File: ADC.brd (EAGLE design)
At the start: 132.1 x 82.5 mm, 368 parts, among them IC1 AD8221ARZ, IC10 AD8605ARTZ, IC11 AD8221ARZ, IC12 TLC2254ID, IC13 AD8605ARTZ, IC14 AD8221ARZ, IC15 TLC2254ID, IC16 AD8605ARTZ, IC17 AD8221ARZ, IC18 TLC2254ID, IC19 AD8605ARTZ, IC2 TLC2254ID, IC20 AD8221ARZ, IC21 TLC2254ID, IC22 AD8605ARTZ, IC23 AD8221ARZ, IC24 TLC2254ID, IC25 AD8605ARTZ, IC26 AD8221ARZ, IC27 TLC2254ID, IC28 AD8605ARTZ, IC3 ADS1256IDBT, IC4 AD8605ARTZ, IC5 MCP170333MB, IC6 ADUM1402ARWZ, IC7 REF3125AIDBZT, IC8 AD8221ARZ, IC9 TLC2254ID, Q1 8MHz

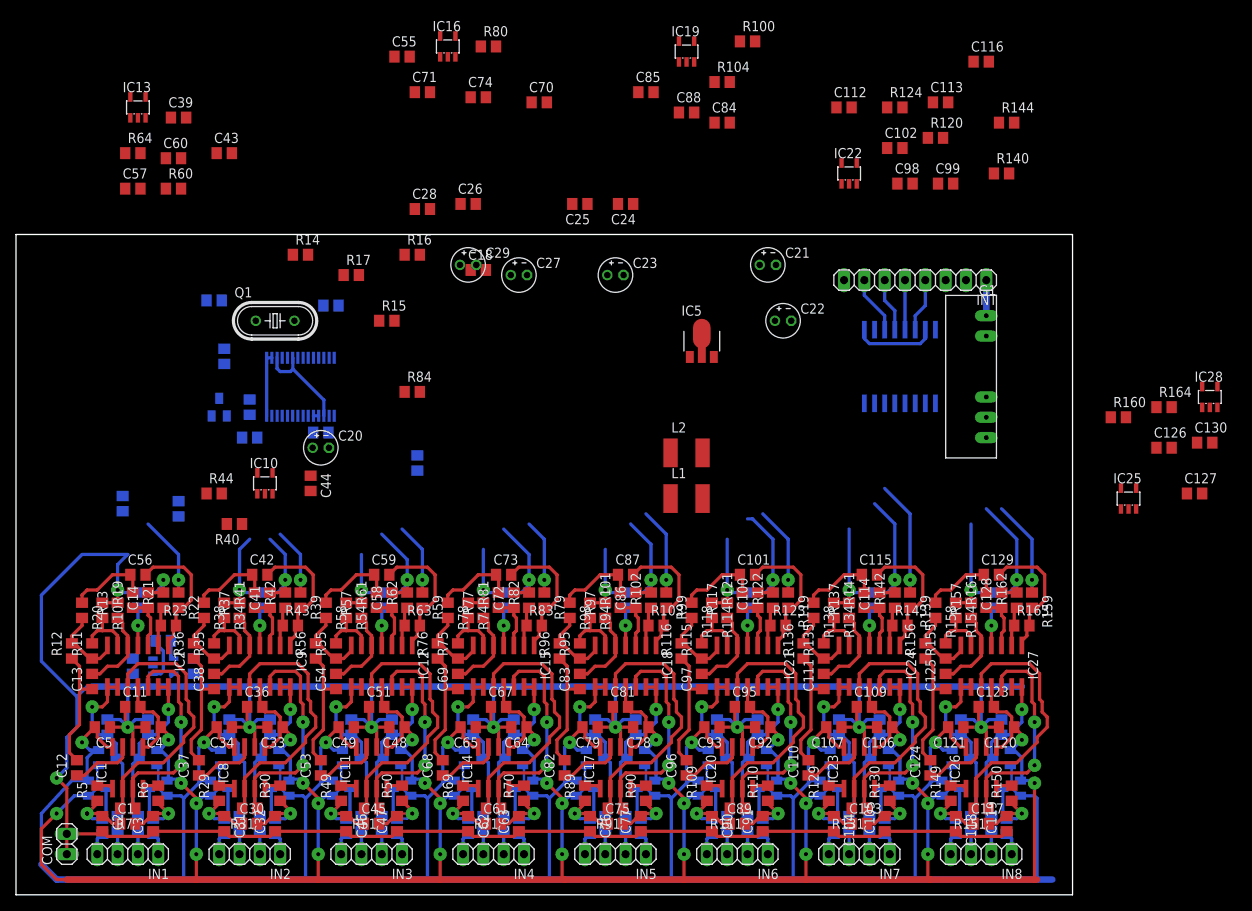
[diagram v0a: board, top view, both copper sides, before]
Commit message: Latest modification for all-in-one board
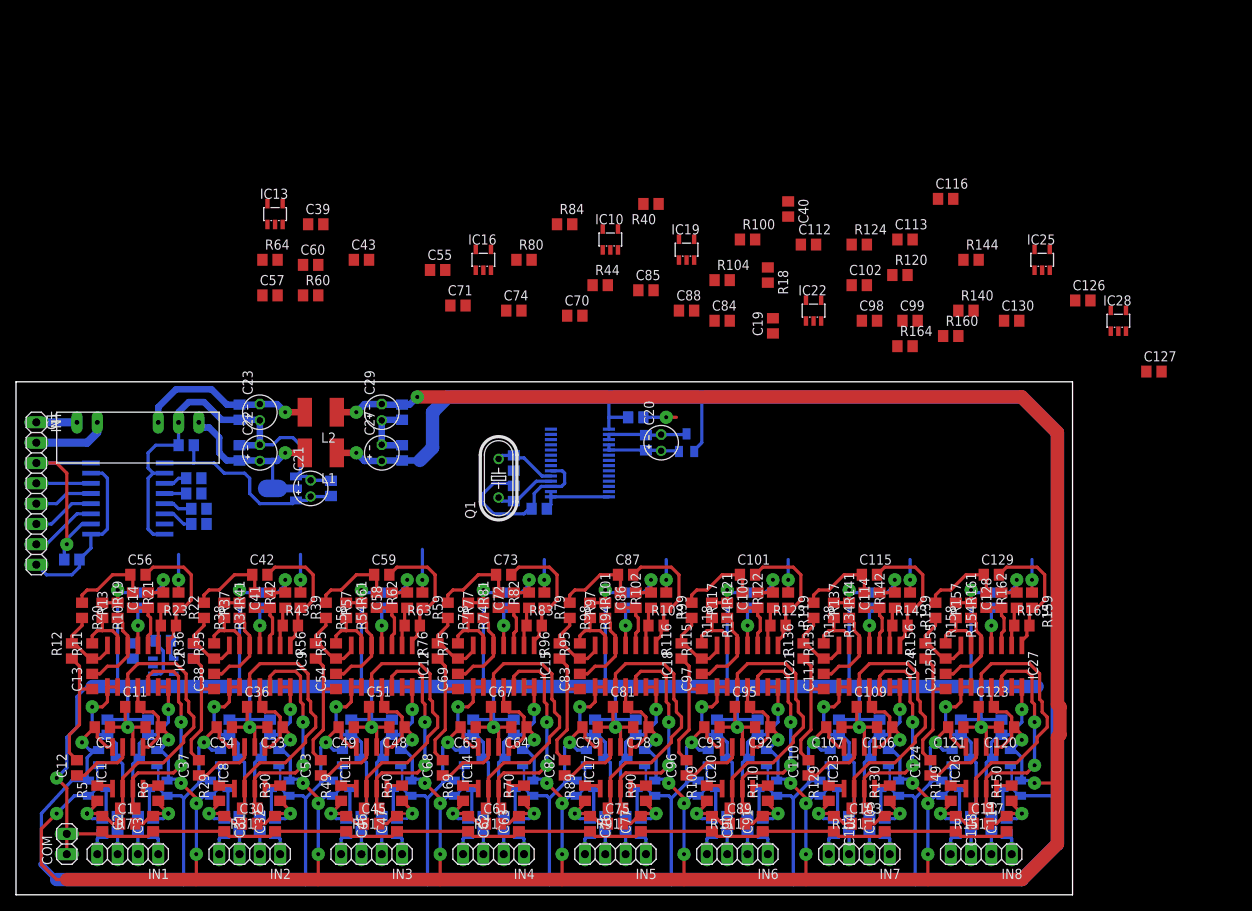
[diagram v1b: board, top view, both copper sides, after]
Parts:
- moved INT 113.0 mm to (2.54, 50.2), turned to 270 degrees
- moved G1 106.2 mm to (15.2, 59.1), turned to 90 degrees
- moved IC6 97.9 mm to (14.0, 49.5), turned to 270 degrees
- moved C19 84.3 mm to (94.6, 71.1), flipped to the top
- moved R18 79.2 mm to (94.0, 77.5), flipped to the top
- moved C22 67.5 mm to (30.5, 55.2), turned to 90 degrees
- moved R40 65.7 mm to (79.4, 86.4)
- moved C21 63.6 mm to (36.8, 50.8), turned to 90 degrees
- moved C18 62.4 mm to (6.99, 41.9), flipped to the bottom, turned to 180 degrees
- moved IC7 58.6 mm to (83.8, 56.5)
- moved C24 57.4 mm to (27.9, 55.2), flipped to the bottom, turned to 90 degrees
- moved C40 56.2 mm to (96.5, 85.7), flipped to the top, turned to 270 degrees
- moved IC5 55.8 mm to (33.0, 50.8), flipped to the bottom, turned to 270 degrees
- moved R44 54.8 mm to (73.0, 76.2)
- moved IC10 52.9 mm to (74.3, 81.9)
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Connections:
- new net N$207: G1.2, INT.2
- net N$37: no longer G1.2, INT.3
- net N$38: now also INT.3; no longer INT.2
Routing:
- net +5VA: track 458.4 -> 616.0 mm, vias 16 -> 17
- net -5VA: track 460.6 -> 599.9 mm, vias 31 -> 33
- net GND: track 685.2 -> 730.5 mm, vias 25 -> 26
- net +3.3V: track 7.90 -> 36.2 mm
- net N$38: track 0.00 -> 26.5 mm, vias 0 -> 1
- net N$44: track 0.00 -> 22.4 mm, vias 0 -> 1
- net N$39: track 0.00 -> 20.2 mm, vias 0 -> 1
- net N$37: track 10.4 -> 22.0 mm
- net N$178: track 14.3 -> 4.13 mm
- net N$207: track 0.00 -> 9.42 mm
- net VREF: track 0.65 -> 9.49 mm
- net N$202: track 12.1 -> 4.13 mm
- net N$13: track 0.00 -> 7.78 mm
- net N$12: track 0.00 -> 7.75 mm
- net N$155: track 11.2 -> 4.13 mm
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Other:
- board size 132.1 x 82.5 mm -> 132.1 x 64.1 mm
